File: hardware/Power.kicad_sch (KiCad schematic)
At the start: 24 parts, among them J200 Conn_Receptacle_2P, Q200 AO3401A, U200 RT9080-33GJ5, U201 TPS61023DRLR, U202 MCP73831-2-OT, X200 12401598E4#2A

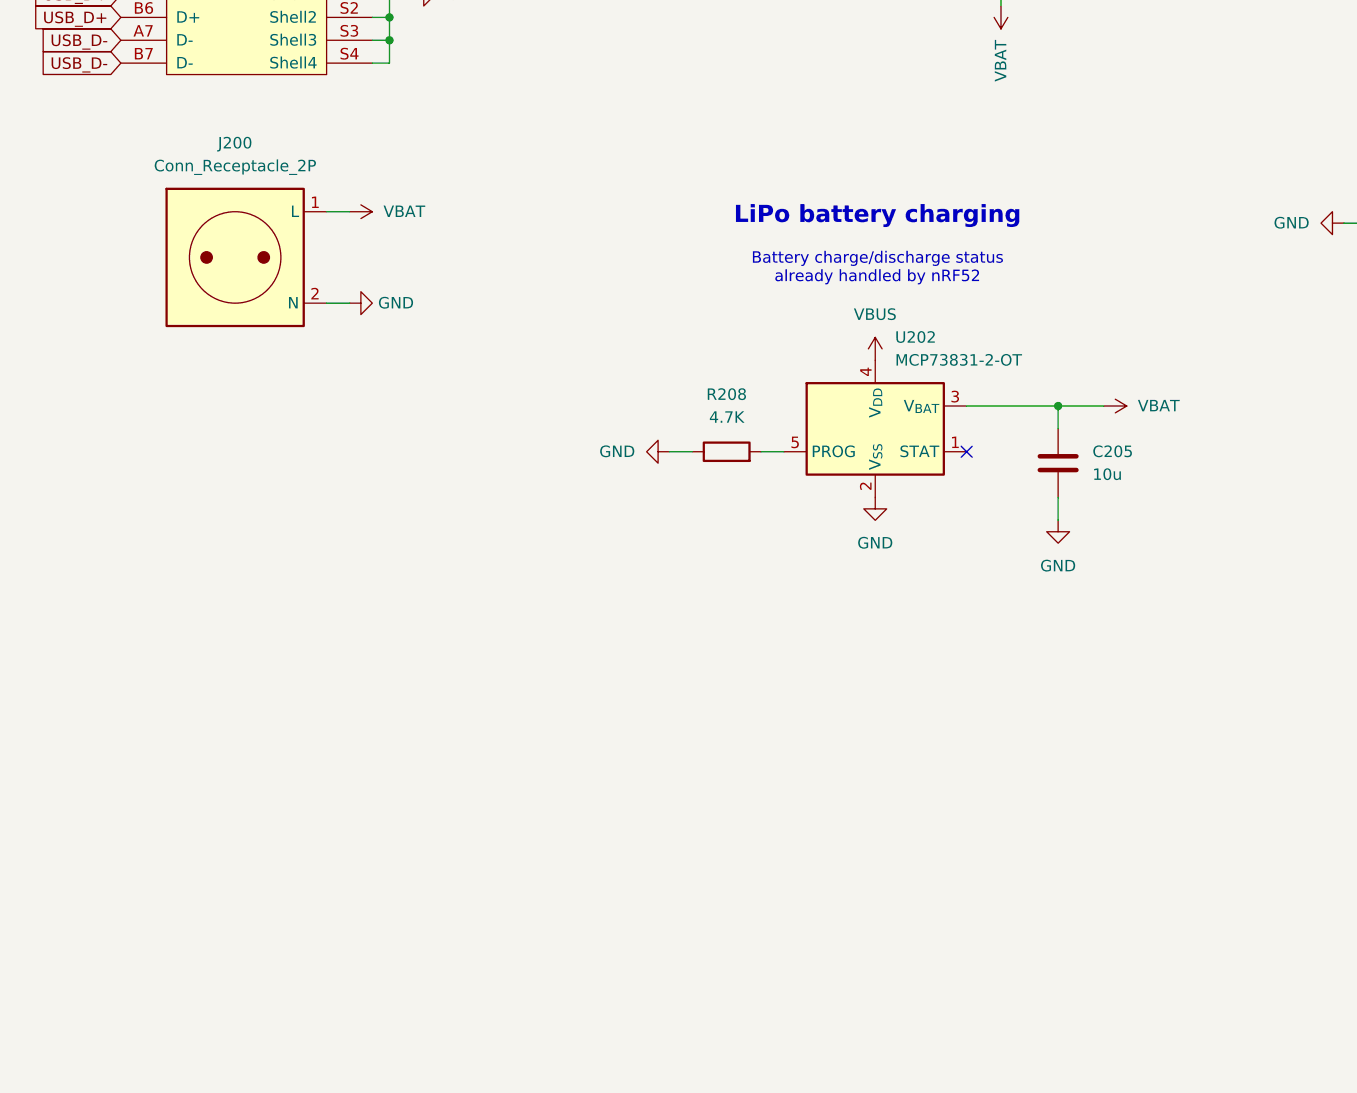
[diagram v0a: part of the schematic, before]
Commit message: Add buttons to PCB layout
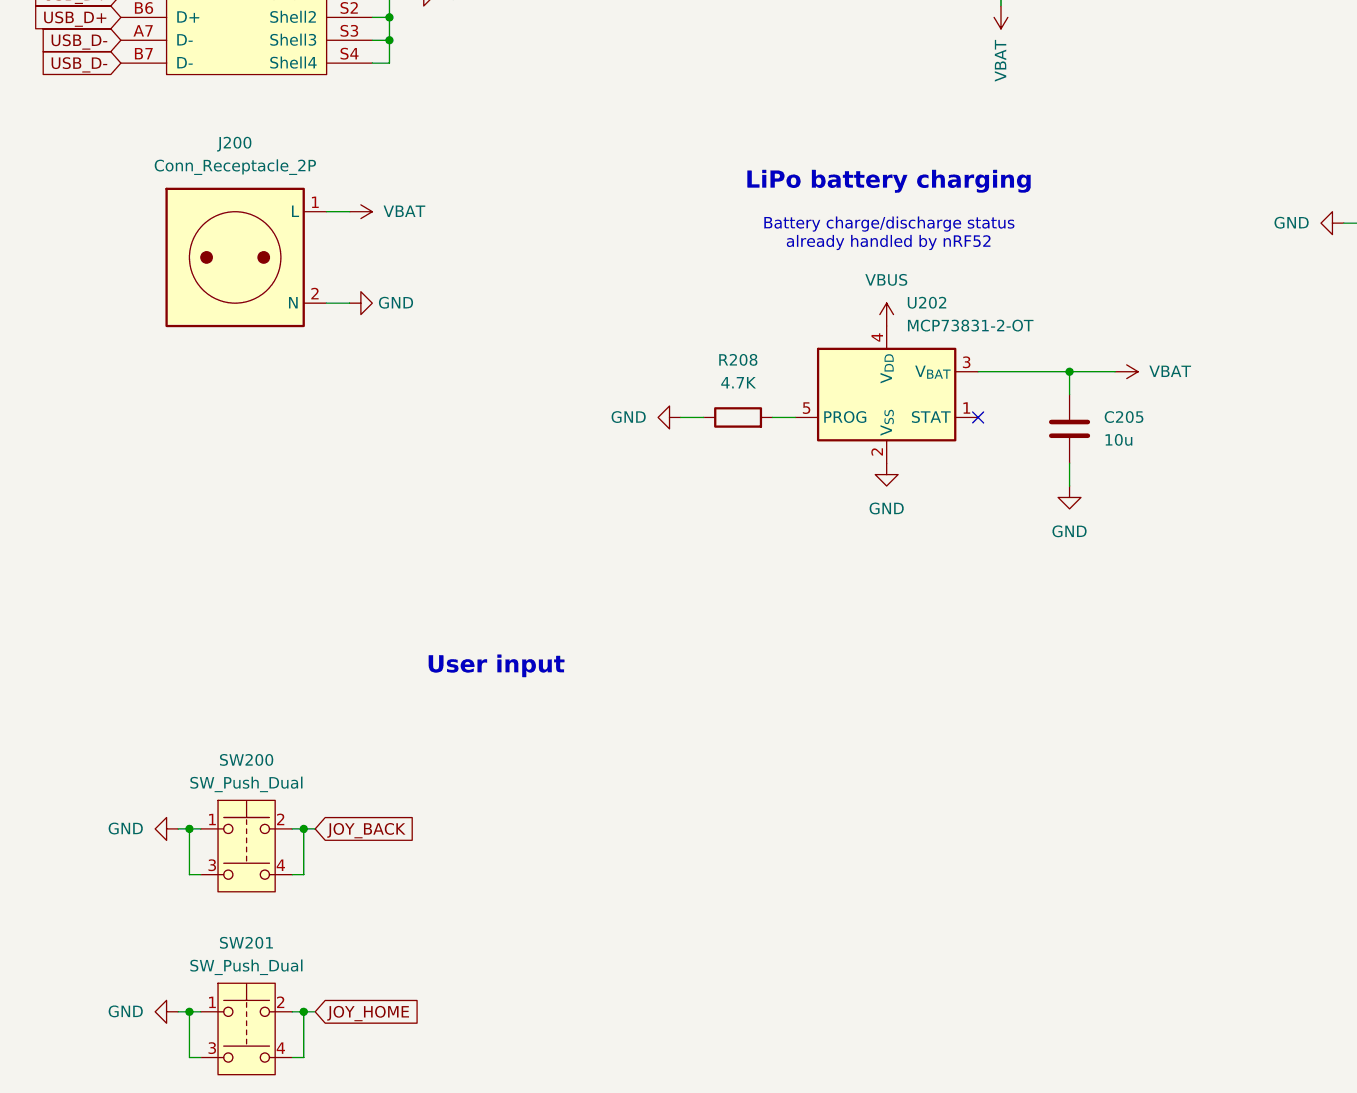
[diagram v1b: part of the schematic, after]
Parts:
- added SW200, SW201: SW_Push_Dual, SMD_SW_6mm:SW_Push_1P1T_NO_6x6mm_H9.5mm, symbol Switch:SW_Push_Dual
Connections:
- net GND: now also SW200.1, SW200.3, SW201.1, SW201.3
- new net JOY_BACK: SW200.2, SW200.4
- new net JOY_HOME: SW201.2, SW201.4
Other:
- note added: "User input"
- moved on the sheet: C205, R208, U202
